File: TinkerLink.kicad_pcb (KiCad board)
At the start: 2 copper layers, 40 x 20 mm, 19 parts, among them J1 Conn_01x06_Pin, Q1 IRF4905S, Q2 MMBT2222A, SW1 TS-061D-250D4-P, U1 ESP-01F-2M, U2 ME6211C33M5

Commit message: fiddlin' with silscreen
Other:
- board text added: "${TITLE} rev. ${REVISION}"
- board text removed: "TinkerLink rev. 0.0.2"
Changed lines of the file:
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@@
 	)
 	(paper "A4")
+	(title_block
+		(title "TinkerLink")
+		(rev "0.0.2")
+	)
 	(layers
 		(0 "F.Cu" signal)
@@
 		)
 	)
-	(gr_text "TinkerLink\nrev. 0.0.2"
+	(gr_text "${TITLE}\nrev. ${REVISION}"
 		(at 108.62 91.5 0)
 		(layer "B.SilkS")

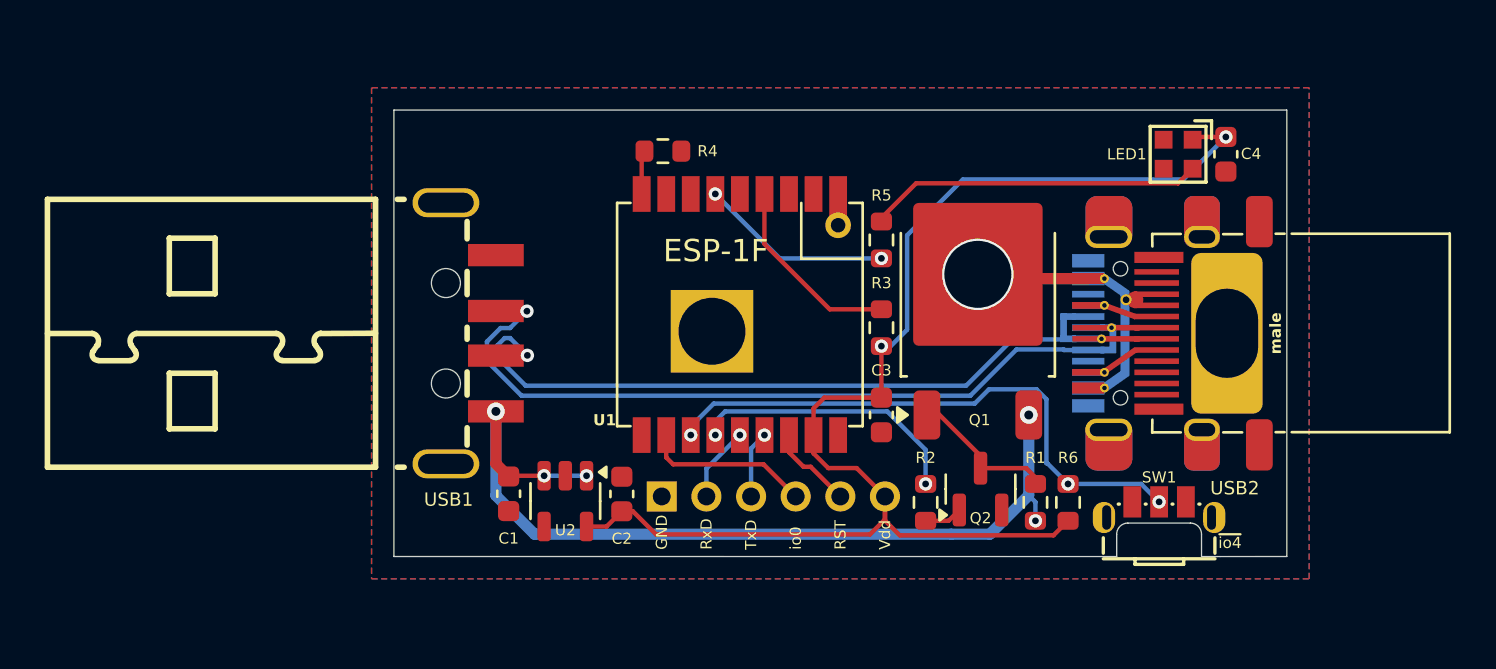
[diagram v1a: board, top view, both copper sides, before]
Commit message: Bloody Rabbit Hole Sub-Basement!
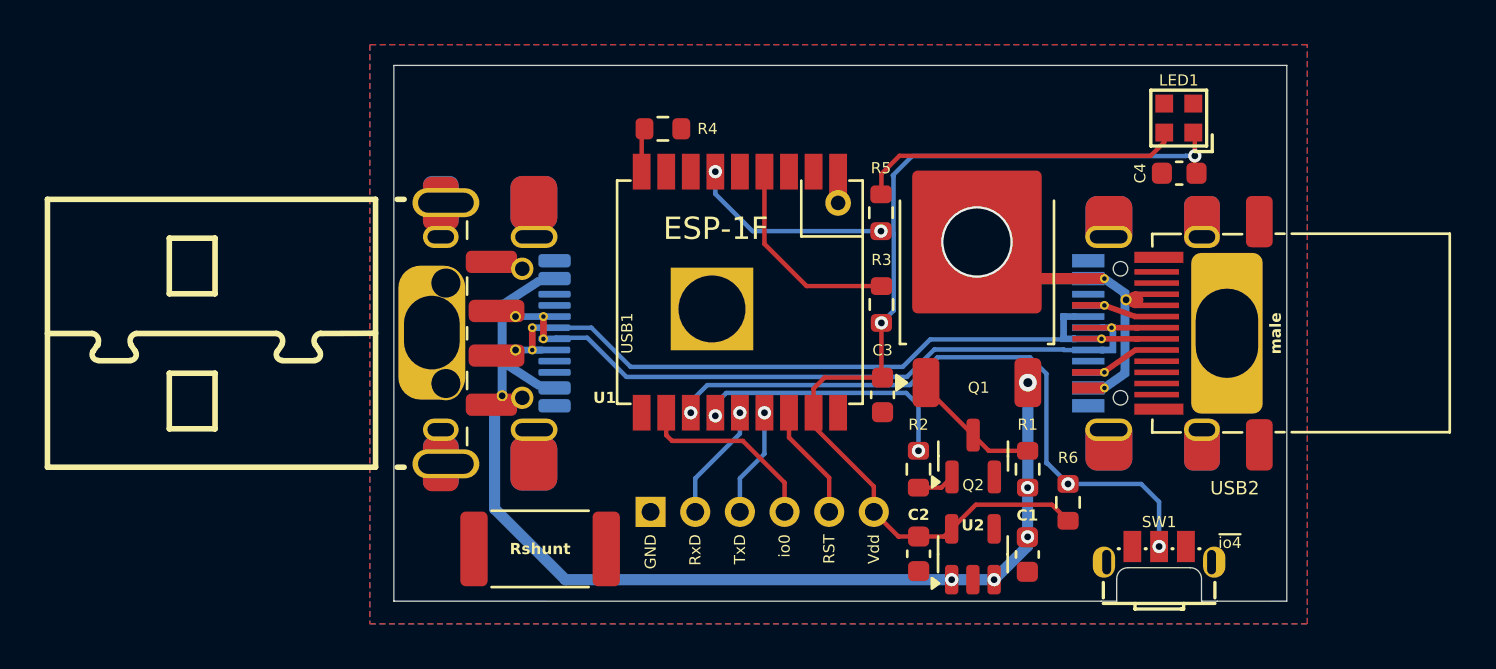
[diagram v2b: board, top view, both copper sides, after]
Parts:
- added Rshunt: 0R1 1%, Resistor_SMD:R_2512_6332Metric, F.Cu at (86.5, 109.7)
- USB1: value USB-212-BCW -> USB-A-USB-C; footprint LCSCfootprints:USB-A-SMD_USB-212-BCW -> tinker:USB-A-USB-C
- moved C1 23.4 mm to (108.4, 109.9)
- moved U2 18.4 mm to (105.9, 109.9), turned to 90 degrees
- moved C2 13.6 mm to (103.5, 109.9), turned to -90 degrees
- moved C4 2.26 mm to (115.2, 92.8), turned to 180 degrees
- moved SW1 2.00 mm to (114.3, 110.0)
- moved LED1 1.62 mm to (115.2, 90.4), turned to 0 degrees
- moved R1 1.53 mm to (108.4, 106.1)
- moved R2 1.52 mm to (103.5, 106.1)
- moved Q2 1.52 mm to (106.0, 105.5)
- moved Q1 1.45 mm to (106.1, 97.2)
- moved R5 1.22 mm to (101.8, 94.6)
- moved R3 1.04 mm to (101.8, 98.7)
- moved R4 1.00 mm to (92.0, 90.8)
- moved U1 1.00 mm to (95.5, 98.2)
- moved C3 0.90 mm to (101.9, 102.8)
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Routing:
- net Vdd: track 60.1 -> 45.2 mm
- net /D+: track 31.7 -> 25.2 mm, vias 1 -> 0
- net /D-: track 30.2 -> 25.3 mm, vias 1 -> 0
- net io4: track 25.8 -> 29.3 mm
- net /Vbus: track 40.6 -> 38.3 mm
- net /VbusS: track 10.0 -> 12.2 mm
- net /Rx: track 3.37 -> 5.33 mm
- net /Tx: track 3.00 -> 4.90 mm
- net /RST: track 3.89 -> 5.19 mm
- net /io0: track 7.52 -> 8.49 mm
- net Net-(Q1-G): track 6.81 -> 5.96 mm
- net /EN: track 8.69 -> 9.26 mm
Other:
- board size 40 x 20 mm -> 40 x 24 mm
